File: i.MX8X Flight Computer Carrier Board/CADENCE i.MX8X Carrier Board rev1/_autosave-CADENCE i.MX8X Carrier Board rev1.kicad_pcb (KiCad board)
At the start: 6 copper layers, 167.7 x 85 mm, 431 parts, among them CN1 DF11-16DP-2DSA(08), CN2 DF11-16DP-2DSA(08), CN3 DF11-16DP-2DSA(08), CN4 DF11-16DP-2DSA(08), J1 BTH-070-02-L-D-A, J10 Conn_01x04, J11 Conn_01x04, J16 Conn_01x04, J17 Conn_01x04, J2 USB_C_Receptacle_USB2.0_16P, J21 Conn_02x02_Odd_Even, J22 Conn_01x04, J3 USB_A, J4 Conn_Coaxial, J5 USB_C_Receptacle_USB2.0_16P, J6 Conn_01x01, J7 Conn_01x08, J8 Conn_02x26_Odd_Even, J9 Conn_02x26_Odd_Even, Q1 IRLML6401, Q2 BSS138, Q3 BSS138, SW1 SW_DIP_x01, SW2 KMR221GLFS, SW3 SW_DIP_x04, SW4 SW_DIP_x01, T1 WE-RJ45_7499111121A, T2 WE-RJ45_7499111121A, U1 LT8612, U10 ZDSD04GLGEAG, U11 MR20H40, U12 MR20H40, U13 DP83867IRRGZR, U14 74LVC2G07, U15 USBLC6-2SC6, U16 USBLC6-2SC6, U17 SN65C1168ERGYR, U18 P82B715DR, U19 P82B715DR, U2 LT8612, U20 P82B715DR, U21 INA219AxDCN, U22 Skytraq Orion B16 GPS, U23 RV-3028-C7, U24 LSM6DSO, U25 LIS2MDL, U26 TMP112xxDRL, U27 INA219AxDCN, U28 LP38693MP-ADJ/NOPB, U29 74CBTLV3257BQ, U3 TPS22975, U30 CAT93C66VI-GT3, U31 USBLC6-2SC6, U32 FT2232HL, U33 SN65HVD233, U34 INA219AxDCN, U35 TPS22810DBV, U36 INA219AxDCN, U37 TPS22810DBV, U38 INA219AxDCN, U39 TPS22975, U4 LT3115-1, U40 TXS0101DCKR, U41 TXS0101DCKR, U5 TLV71325PDQNR, U6 TLV71310PDQNR, U7 TLV1704, U8 BD2204GUL-E2, U9 MX25UM51245G, Y1 25MHz, Y2 12MHz

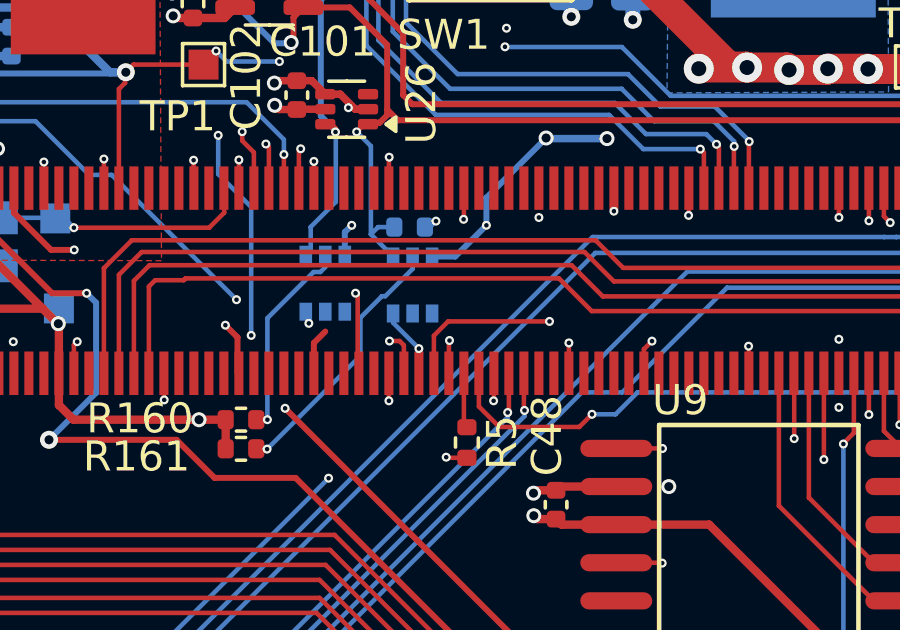
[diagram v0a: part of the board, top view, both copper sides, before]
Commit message: DRC fixes
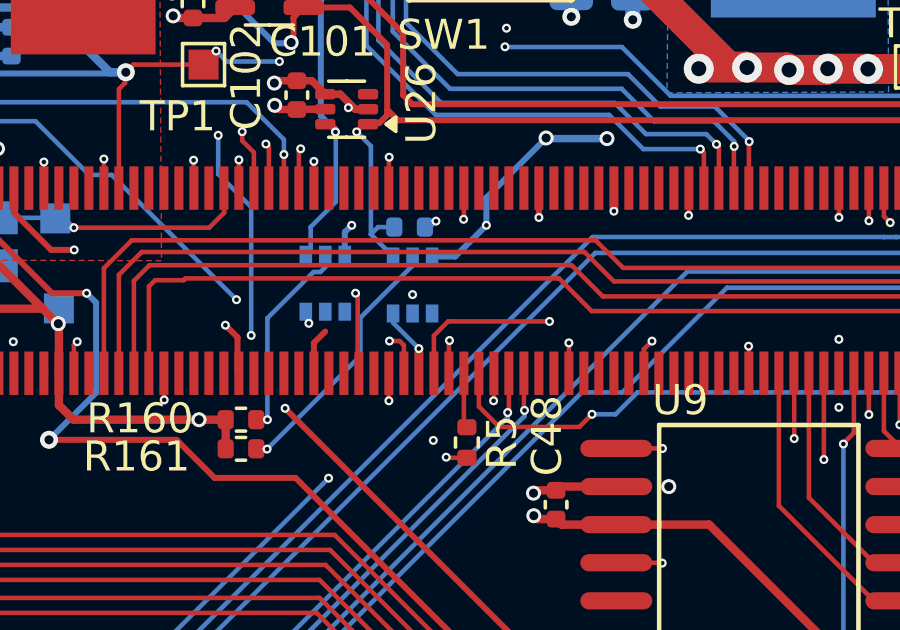
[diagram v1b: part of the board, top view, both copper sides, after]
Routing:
- net GND: track 287.6 -> 288.6 mm, vias 384 -> 386
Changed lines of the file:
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@@
 	)
 	(segment
+		(start 292.61 93.92)
+		(end 292.61 92.94)
+		(width 0.2)
+		(layer "F.Cu")
+		(net 1)
+	)
+	(segment
 		(start 352.7275 105.39)
 		(end 351.777488 105.39)
@@
 	)
 	(via
+		(at 289.09 101.35)
+		(size 0.3)
+		(drill 0.15)
+		(layers "F.Cu" "B.Cu")
+		(free yes)
+		(net 1)
+	)
+	(via
 		(at 343.62 95.18)
 		(size 0.6)
@@
 	)
 	(via
+		(at 288.4 96.49)
+		(size 0.3)
+		(drill 0.15)
+		(layers "F.Cu" "B.Cu")
+		(free yes)
+		(net 1)
+	)
+	(via
 		(at 345.75 135.7)
 		(size 0.3)
@@
 	)
 	(segment
-		(start 283.55 101.64)
-		(end 286.66 98.53)
-		(width 0.1525)
-		(layer "B.Cu")
-		(net 574)
-	)
-	(segment
-		(start 287.49175 96.54275)
-		(end 288.4 95.6345)
-		(width 0.1525)
-		(layer "B.Cu")
-		(net 574)
-	)
-	(segment
 		(start 286.66 98.53)
 		(end 286.66 97.26)
@@
 	)
 	(segment
-		(start 287.37725 96.54275)
-		(end 287.49175 96.54275)
+		(start 288.4 95.52)
+		(end 288.4 95.22)
 		(width 0.1525)
 		(layer "B.Cu")
@@
 	)
 	(segment
-		(start 288.4 95.6345)
-		(end 288.4 95.22)
+		(start 286.66 97.26)
+		(end 288.4 95.52)
 		(width 0.1525)
 		(layer "B.Cu")
@@
 	)
 	(segment
-		(start 286.66 97.26)
-		(end 287.37725 96.54275)
+		(start 283.55 101.64)
+		(end 286.66 98.53)
 		(width 0.1525)
 		(layer "B.Cu")
